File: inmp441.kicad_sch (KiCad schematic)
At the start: 7 parts

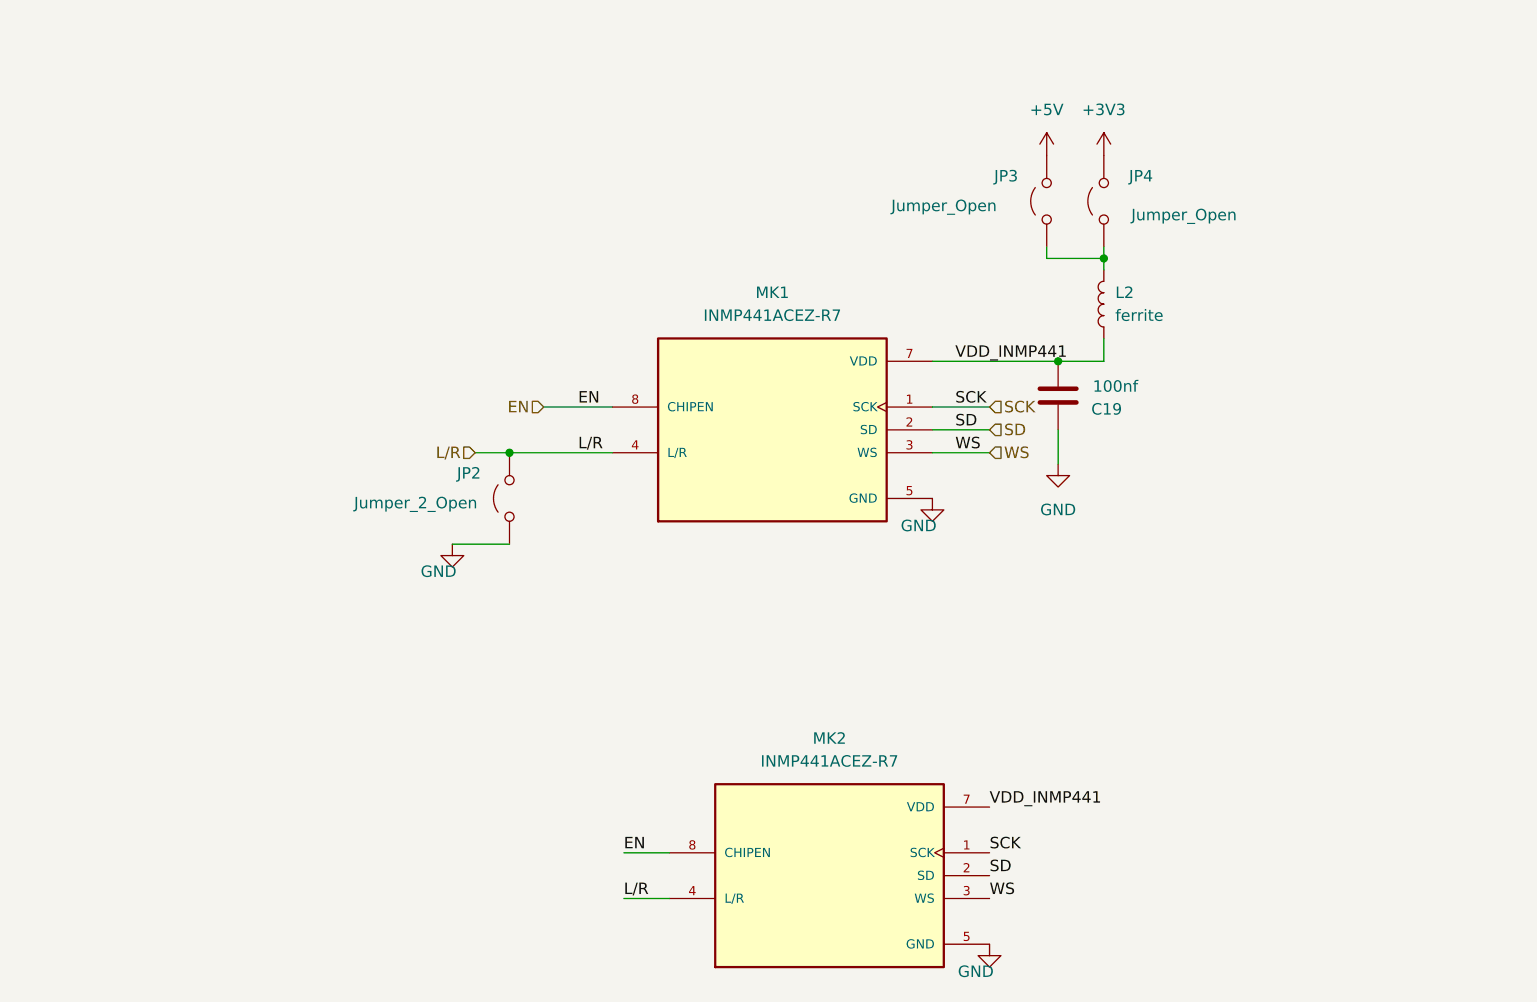
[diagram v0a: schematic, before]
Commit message: Update all schematic files and project
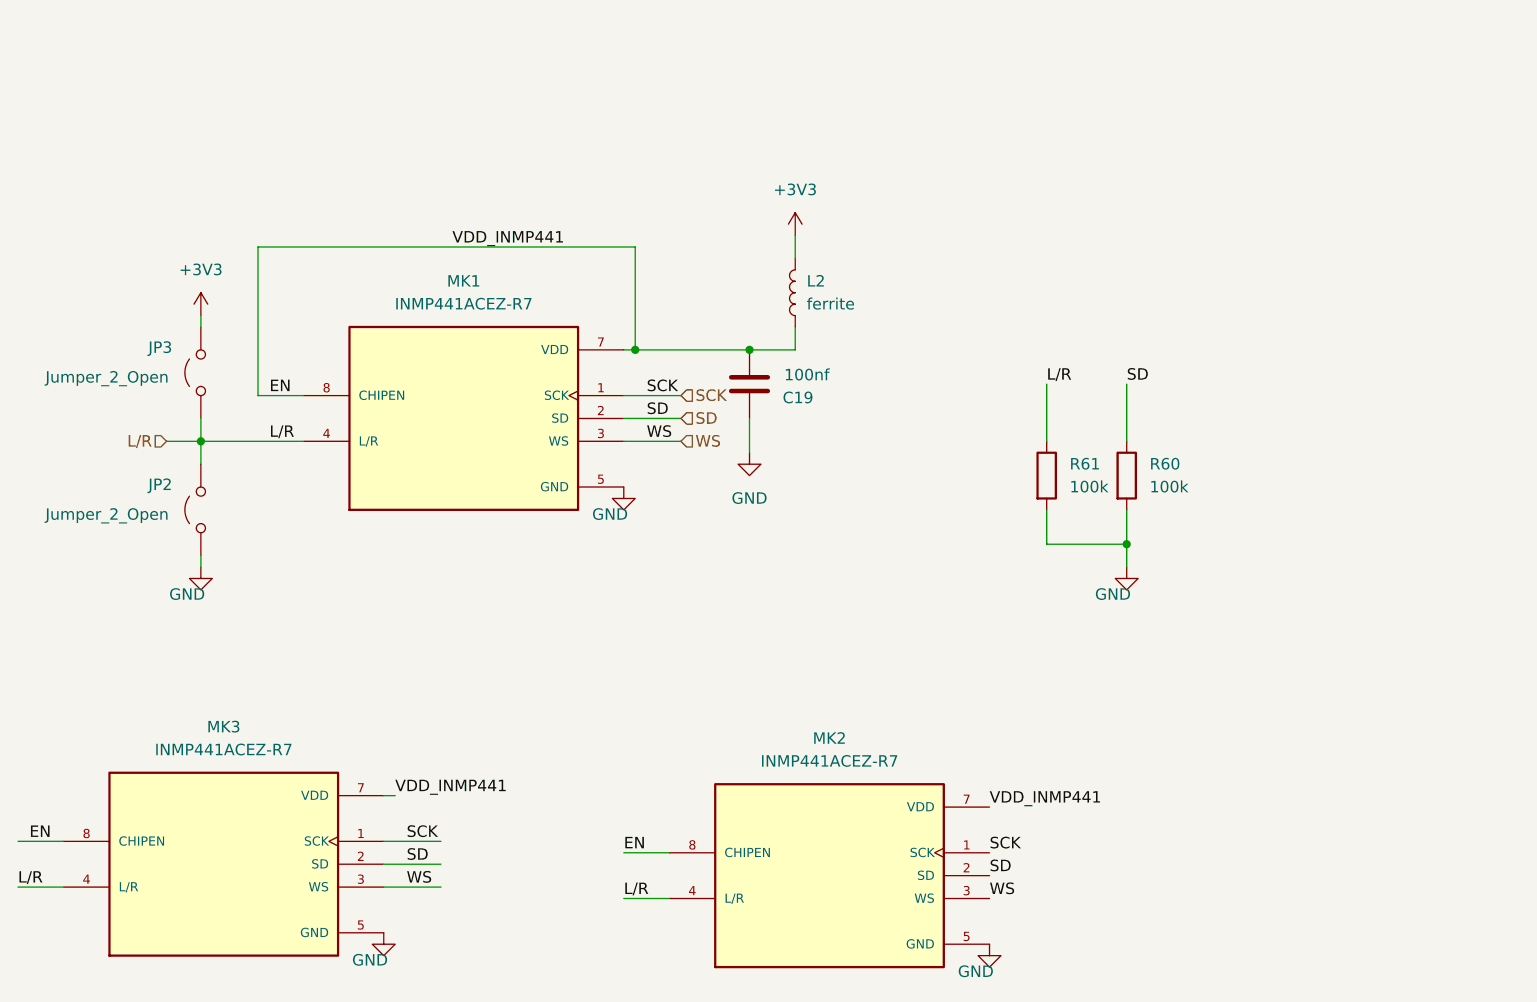
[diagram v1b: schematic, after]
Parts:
- removed JP4: Jumper_Open, Jumper:SolderJumper-2_P1.3mm_Open_RoundedPad1.0x1.5mm, symbol Jumper:Jumper_2_Open
- added MK3: INMP441ACEZ-R7, kiC:MIC_INMP441ACEZ-R7, symbol INMP441ACEZ-R7:INMP441ACEZ-R7
- added R60, R61: 100k, Resistor_SMD:R_0805_2012Metric, symbol Device:R
- JP3: value Jumper_Open -> Jumper_2_Open
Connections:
- net +5V is gone; now on net +3V3: JP3.2 (B)
- net VDD_INMP441 is gone; now on net EN: C19.2, L2.1, MK1.7 (VDD), MK2.7 (VDD)
- net +3V3: now also L2.2
- net EN: now also MK3.7 (VDD), MK3.8 (CHIPEN)
- net GND: now also MK3.5 (GND), MK3.6 (GND), MK3.9 (GND), R60.2, R61.2
- net L/R: now also JP3.1 (A), MK3.4 (L/R), R61.1
- net SCK: now also MK3.1 (SCK)
- net SD: now also MK3.2 (SD), R60.1
- net WS: now also MK3.3 (WS)
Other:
- moved on the sheet: C19, JP2, L2, MK1

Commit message: Update all schematic files and project
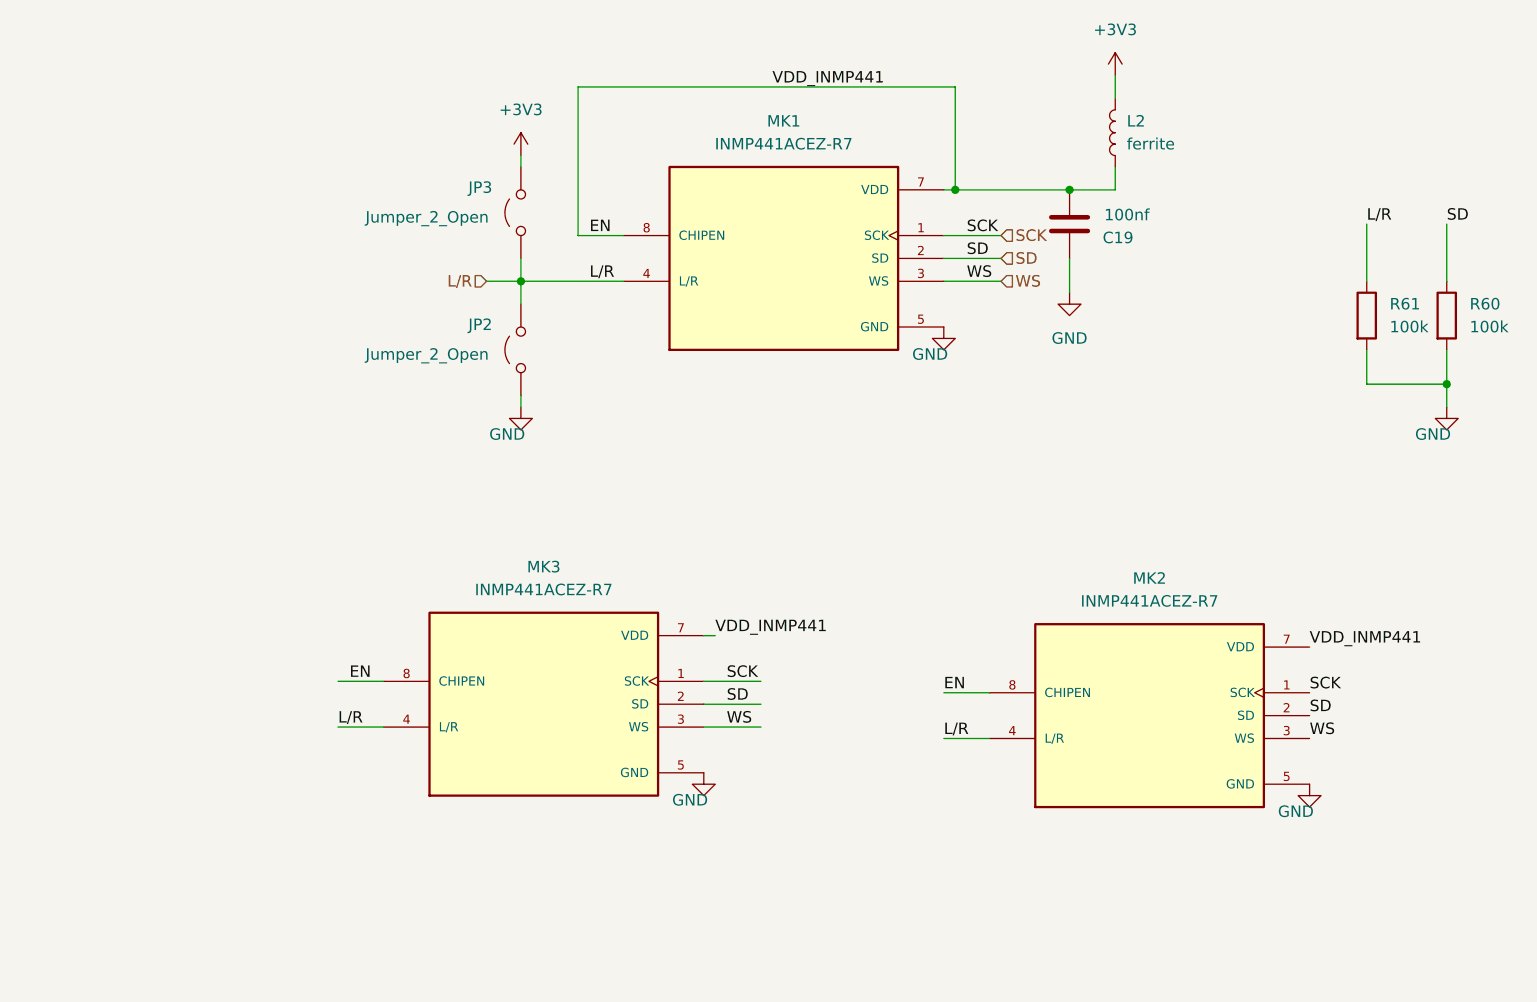
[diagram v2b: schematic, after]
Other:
- moved on the sheet: C19, JP2, JP3, L2, MK1, MK2, MK3, R60, R61
